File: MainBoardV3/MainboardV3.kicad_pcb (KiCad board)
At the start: 2 copper layers, 100 x 100 mm, 47 parts, among them J1 Conn_01x02, J10 Conn_01x04, J11 Conn_01x02, J12 Conn_01x02, J13 Conn_01x02, J14 Conn_01x02, J15 Conn_01x02, J16 Conn_01x02, J17 Conn_01x02, J18 Conn_01x03, J19 Conn_02x03_Odd_Even, J2 Conn_01x04, J20 Conn_02x03_Odd_Even, J21 Conn_02x03_Odd_Even, J22 Conn_01x03, J23 Conn_01x05, J24 Conn_02x05_Odd_Even, J3 Conn_01x03, J4 Conn_01x04, J5 Conn_01x05, J6 Conn_01x02, J7 Conn_01x04, J8 Conn_01x04, J9 Conn_01x04, U1 TSR_2-2450, U2 ESP32-S3-DevKitC, U3 TSR_2-2433, U4 TEN_50-2411WI

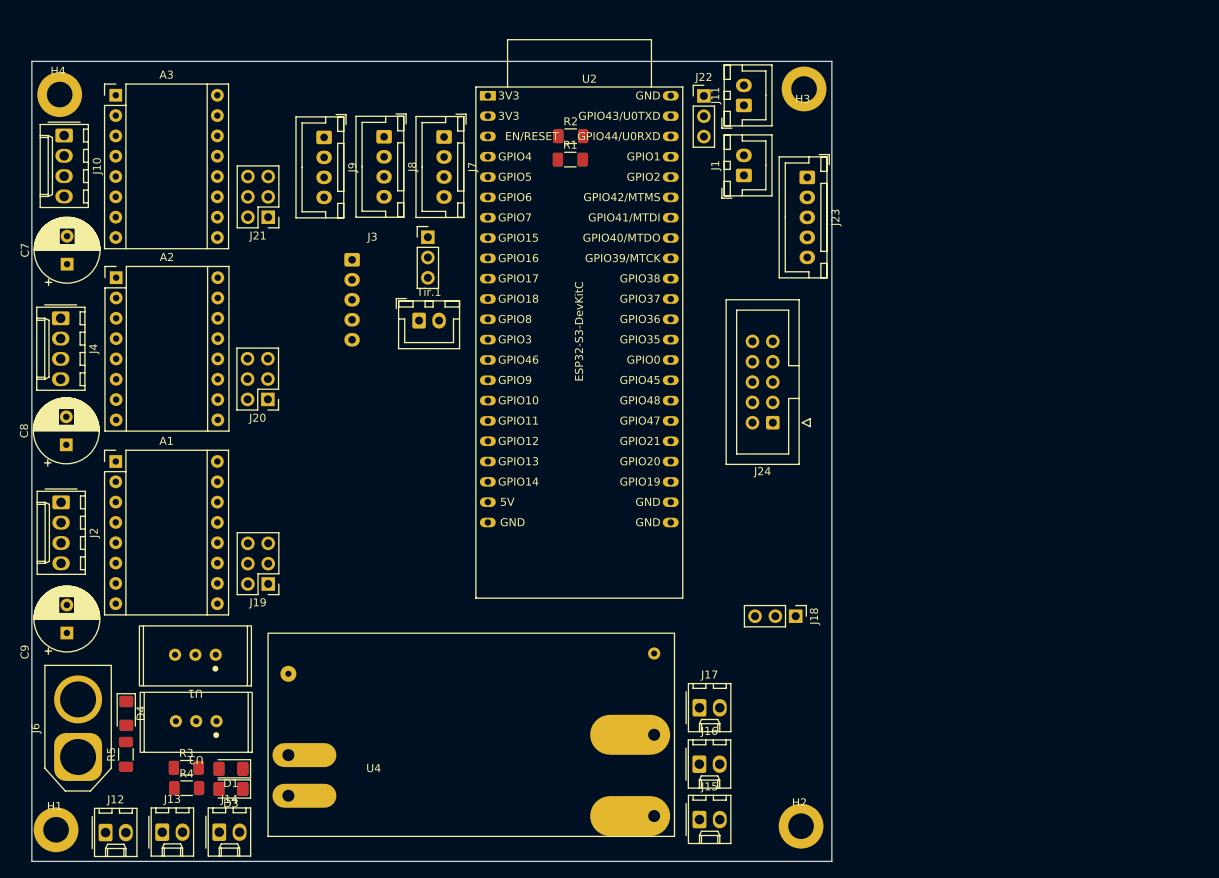
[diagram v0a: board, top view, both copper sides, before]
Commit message: Mise a jour pour remi
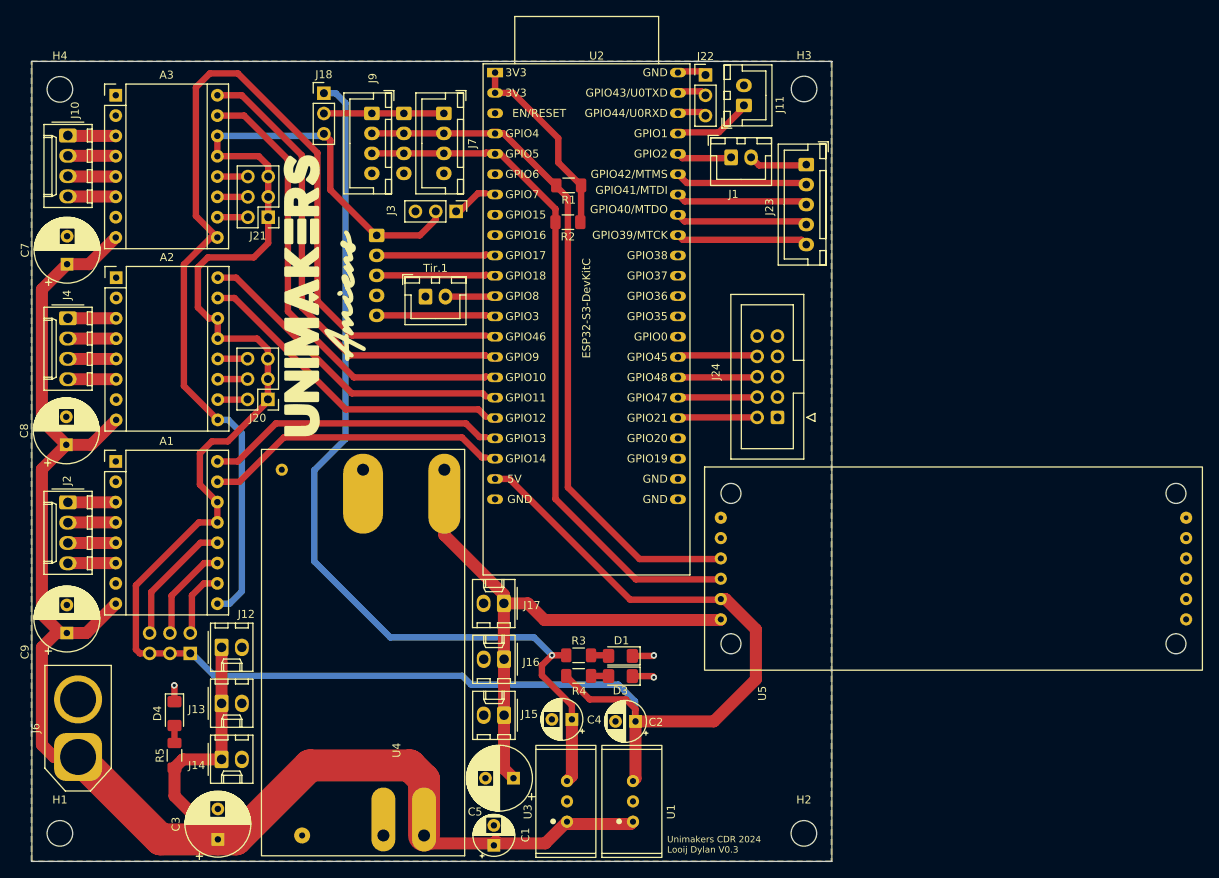
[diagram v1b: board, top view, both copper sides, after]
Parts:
- added C1: C_Polarized, Capacitor_THT:CP_Radial_D5.0mm_P2.50mm, F.Cu at (7.75, 48.0)
- added C2: C_Polarized, Capacitor_THT:CP_Radial_D5.0mm_P2.50mm, F.Cu at (25.5, 32.5)
- added C3: C_Polarized, Capacitor_THT:CP_Radial_D8.0mm_P3.80mm, F.Cu at (-26.8, 47.2)
- added C4: C_Polarized, Capacitor_THT:CP_Radial_D5.0mm_P2.50mm, F.Cu at (17.5, 32.2)
- added C5: C_Polarized, Capacitor_THT:CP_Radial_D8.0mm_P3.50mm, F.Cu at (10.2, 39.6)
- added U5: ~, Custom:PCA9685breakout, F.Cu at (65.2, 13.4)
- H1, H2, H3, H4: footprint MountingHole:MountingHole_3.2mm_M3_DIN965_Pad -> MountingHole:MountingHole_3.2mm_M3
- J19, J8: moved to B.Cu
- moved J18 88.0 mm to (-13.5, -46.0), turned to 0 degrees
- moved U1 57.5 mm to (25.0, 42.5), turned to 90 degrees
- moved R3 51.0 mm to (18.3, 24.2)
- moved R4 51.0 mm to (18.3, 26.8)
- moved D1 50.7 mm to (23.6, 24.3)
- moved D3 50.7 mm to (23.6, 26.8)
- moved U3 47.3 mm to (16.8, 42.5), turned to 90 degrees
- moved J16 27.7 mm to (9.02, 24.7), turned to 180 degrees
- moved J17 27.7 mm to (9.00, 17.8), turned to 180 degrees
- moved J15 27.7 mm to (9.02, 31.7), turned to 180 degrees
- moved J12 27.3 mm to (-26.3, 23.2)
- moved J13 17.7 mm to (-26.3, 30.2)
- moved U4 16.8 mm to (-8.50, 24.0), turned to 90 degrees
- moved J19 13.0 mm to (-30.2, 24.0), turned to 90 degrees
- moved R2 10.8 mm to (17.0, -29.9), turned to 180 degrees
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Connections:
- J24 pad 10: unconnected-(J24-Pin_10-Pad10) -> GND
- J24 pad 2: unconnected-(J24-Pin_2-Pad2) -> GPIO21
- J24 pad 3: unconnected-(J24-Pin_3-Pad3) -> GPIO38
- J24 pad 4: unconnected-(J24-Pin_4-Pad4) -> GPIO47
- J24 pad 5: unconnected-(J24-Pin_5-Pad5) -> GPIO37
- J24 pad 6: unconnected-(J24-Pin_6-Pad6) -> GPIO48
- J24 pad 7: unconnected-(J24-Pin_7-Pad7) -> GPIO36
- J24 pad 8: unconnected-(J24-Pin_8-Pad8) -> GPIO45
- J24 pad 9: unconnected-(J24-Pin_9-Pad9) -> GPI035
- J3 pad 1: +5V -> Neopixel
- J3 pad 2: Neopixel -> +5V
- U2 pad 27: unconnected-(U2-GPIO21-Pad27) -> GPIO21
- U2 pad 28: unconnected-(U2-GPIO47-Pad28) -> GPIO47
- U2 pad 29: unconnected-(U2-GPIO48-Pad29) -> GPIO48
- U2 pad 30: unconnected-(U2-GPIO45-Pad30) -> GPIO45
- U2 pad 32: unconnected-(U2-GPIO35-Pad32) -> GPI035
- U2 pad 33: unconnected-(U2-GPIO36-Pad33) -> GPIO36
- U2 pad 34: unconnected-(U2-GPIO37-Pad34) -> GPIO37
- U2 pad 35: unconnected-(U2-GPIO38-Pad35) -> GPIO38
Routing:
- net +5V: track 0.00 -> 284.4 mm
- net +12V: track 0.00 -> 214.2 mm
- net EN: track 0.00 -> 135.2 mm
- net +3.3VP: track 0.00 -> 116.5 mm, vias 0 -> 1
- net SDA: track 0.00 -> 87.0 mm
- net SCL: track 0.00 -> 86.9 mm
- net +5VP: track 0.00 -> 70.2 mm
- net STEP3: track 0.00 -> 58.3 mm
- net DIR3: track 0.00 -> 58.2 mm
- net STEP2: track 0.00 -> 39.7 mm
- net DIR2: track 0.00 -> 39.7 mm
- net STEP1: track 0.00 -> 36.9 mm
- net DIR1: track 0.00 -> 36.2 mm
- net +3.3V: track 0.00 -> 24.5 mm
- net GND: track 0.00 -> 18.6 mm, vias 0 -> 3
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- added copper zone on B.Cu, net GND
- added copper zone on F.Cu, net GND
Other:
- board text added: "Unimakers CDR 2024 Looij Dylan V0.3"
